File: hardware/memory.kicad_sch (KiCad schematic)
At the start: 13 parts, among them U2 ICE40HX4K-TQ144, U3 SN74ALVC164245, U4 SN74ALVC164245, U5 W25Q32JVSSIM

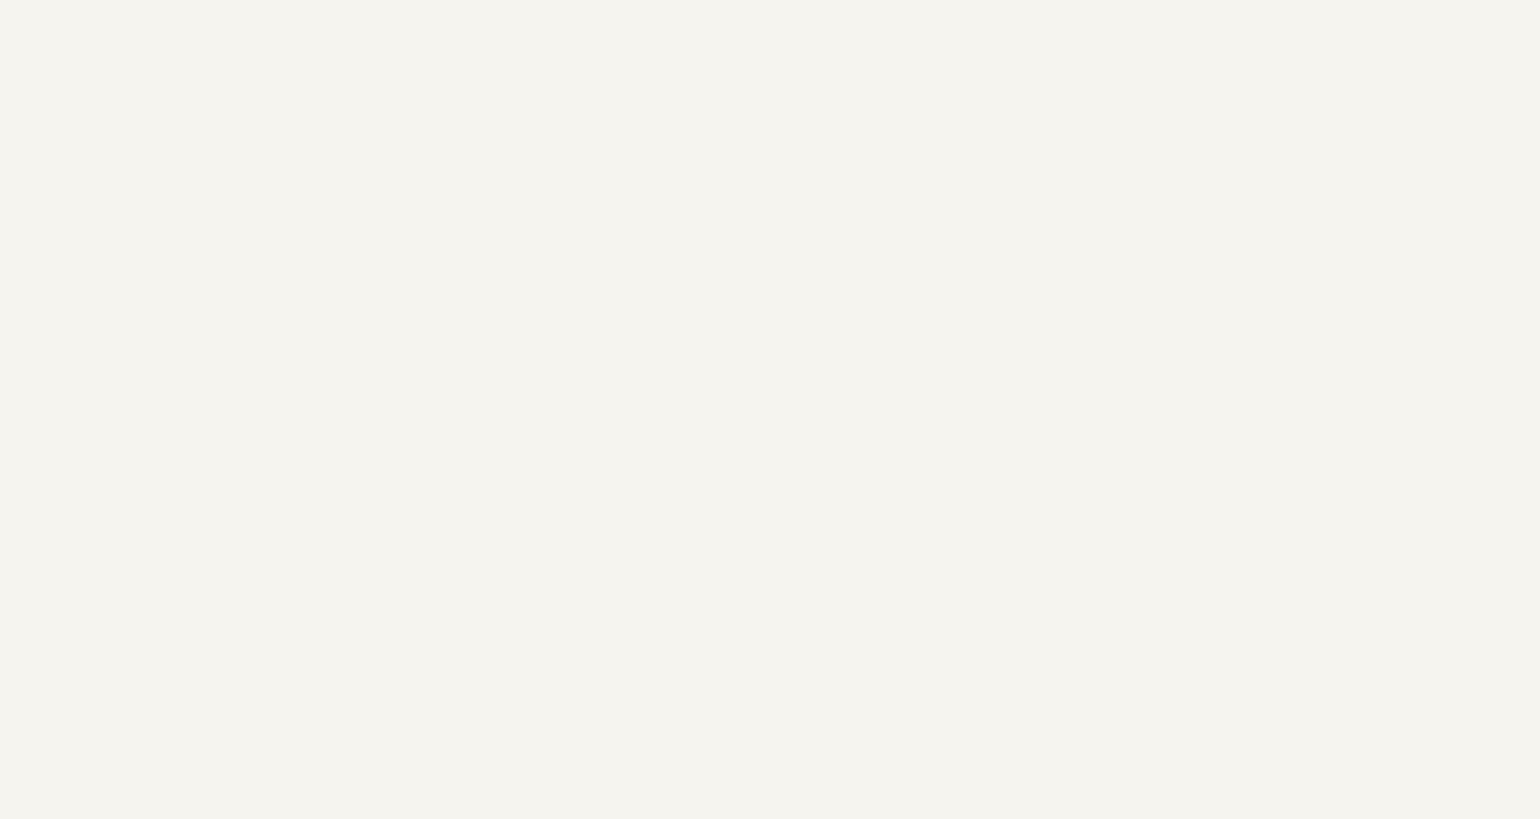
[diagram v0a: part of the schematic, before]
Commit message: updates
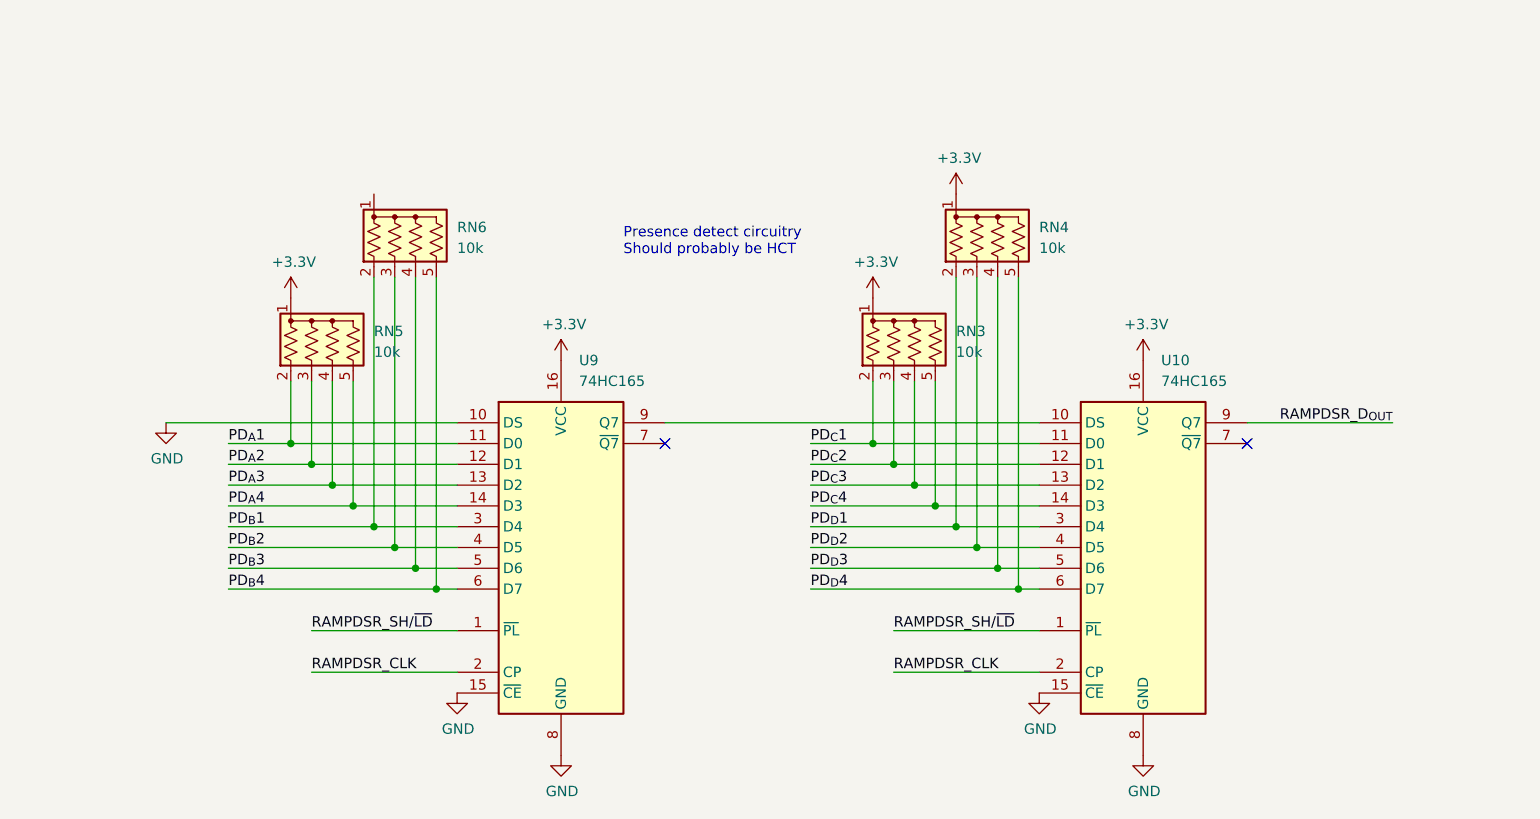
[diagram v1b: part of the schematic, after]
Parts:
- added RN3, RN4, RN5, RN6: 10k, Resistor_THT:R_Array_SIP5, symbol Device:R_Network04_US
- added U10, U9: 74HC165, Package_SO:SOIC-16_3.9x9.9mm_P1.27mm, symbol 74xx:74HC165
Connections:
- net +3V3: now also RN3.1 (common), RN4.1 (common), RN5.1 (common), U10.16 (VCC), U9.16 (VCC)
- net GND: now also U10.15 (~{CE}), U10.8 (GND), U9.10 (DS), U9.15 (~{CE}), U9.8 (GND)
- net PD_{A}1: now also RN5.2 (R1), U9.11 (D0)
- net PD_{A}2: now also RN5.3 (R2), U9.12 (D1)
- net PD_{A}3: now also RN5.4 (R3), U9.13 (D2)
- net PD_{A}4: now also RN5.5 (R4), U9.14 (D3)
- net PD_{B}1: now also RN6.2 (R1), U9.3 (D4)
- net PD_{B}2: now also RN6.3 (R2), U9.4 (D5)
- net PD_{B}3: now also RN6.4 (R3), U9.5 (D6)
- net PD_{B}4: now also RN6.5 (R4), U9.6 (D7)
- net PD_{C}1: now also RN3.2 (R1), U10.11 (D0)
- net PD_{C}2: now also RN3.3 (R2), U10.12 (D1)
- net PD_{C}3: now also RN3.4 (R3), U10.13 (D2)
- net PD_{C}4: now also RN3.5 (R4), U10.14 (D3)
- net PD_{D}1: now also RN4.2 (R1), U10.3 (D4)
- net PD_{D}2: now also RN4.3 (R2), U10.4 (D5)
- net PD_{D}3: now also RN4.4 (R3), U10.5 (D6)
- net PD_{D}4: now also RN4.5 (R4), U10.6 (D7)
- new net: U10.10 (DS), U9.9 (Q7)
- new net RAMPDSR_CLK: U10.2 (CP), U9.2 (CP)
- new net RAMPDSR_D_{OUT}: U10.9 (Q7)
- new net RAMPDSR_SH/~{LD}: U10.1 (~{PL}), U9.1 (~{PL})
- no-connect marks 2 -> 4
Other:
- note added: "Presence detect circuitry Should probably be HCT"
